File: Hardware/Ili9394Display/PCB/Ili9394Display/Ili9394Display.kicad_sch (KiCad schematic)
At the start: 2 parts, among them J1 Conn_01x08_Male, J2 Conn_01x08_Female

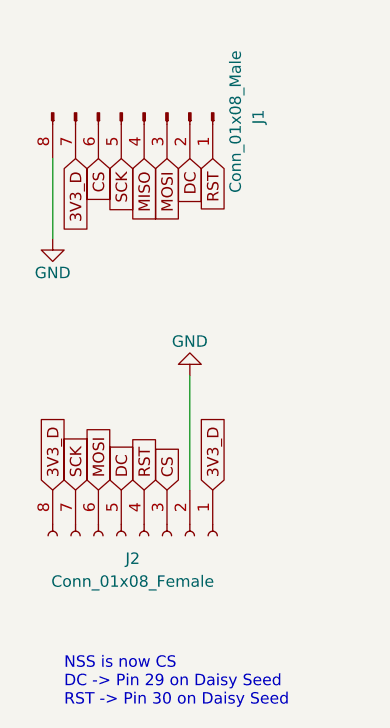
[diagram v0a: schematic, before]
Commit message: Finalised PCBs
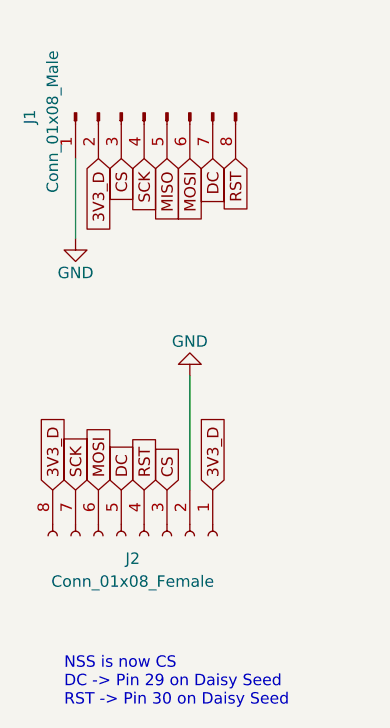
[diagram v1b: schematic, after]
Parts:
- J1: footprint Connector_PinSocket_2.54mm:PinSocket_1x08_P2.54mm_Vertical -> Connector_PinHeader_2.54mm:PinHeader_1x08_P2.54mm_Horizontal
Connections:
- net 3V3_D: now also J1.2 (Pin_2); no longer J1.7 (Pin_7)
- net CS: now also J1.3 (Pin_3); no longer J1.6 (Pin_6)
- net DC: now also J1.7 (Pin_7); no longer J1.2 (Pin_2)
- net GND: now also J1.1 (Pin_1); no longer J1.8 (Pin_8)
- net MISO: now also J1.5 (Pin_5); no longer J1.4 (Pin_4)
- net MOSI: now also J1.6 (Pin_6); no longer J1.3 (Pin_3)
- net RST: now also J1.8 (Pin_8); no longer J1.1 (Pin_1)
- net SCK: now also J1.4 (Pin_4); no longer J1.5 (Pin_5)
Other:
- moved on the sheet: J1
